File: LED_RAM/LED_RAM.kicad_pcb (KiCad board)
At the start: 2 copper layers, 196.3 x 403.9 mm, 91 parts, among them J1 DIN, J10 USB_C_Receptacle_PowerOnly_6P, J12 Conn_01x08_Pin, J13 Conn_01x22_Pin, J14 Conn_01x22_Pin, J15 Conn_01x22_Pin, J16 Conn_01x22_Pin, J2 5V, J3 GND, J4 DOUT, J5 Conn_01x05_Pin, J6 Conn_01x10_Pin, J7 DIN, J8 GND, J9 5V, U1 ER_OLEDM0.91_1x-I2C, U2 ER_OLEDM0.91_1x-I2C, U5 TXS0108EPW, U6 TXS0108EPW, U7 TXS0108EPW

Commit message: Add files via upload
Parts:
- moved D33 290.1 mm to (-33.7, 25.3)
- moved D34 290.1 mm to (-33.7, 50.3)
- moved D35 290.1 mm to (-33.7, 75.3)
- moved D38 290.1 mm to (-33.7, 150.3)
- moved D39 290.1 mm to (-33.7, 175.3)
- moved D40 290.1 mm to (-33.7, 200.3)
- moved J1 290.1 mm to (-46.9, 204.6)
- moved J2 290.1 mm to (46.3, 25.1)
- moved J4 290.1 mm to (-50.5, 204.6)
- moved D1 290.1 mm to (-133.4, 25.2)
- moved D10 290.1 mm to (-108.9, 50.1)
- moved D11 290.1 mm to (-108.9, 75.1)
- moved D12 290.1 mm to (-108.9, 100.1)
- moved D13 290.1 mm to (-108.9, 125.1)
- moved D14 290.1 mm to (-108.9, 150.1)
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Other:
- board size 196.3 x 403.9 mm -> 400.6 x 200.2 mm
- board text added: "SOUP-A COOL LED CUBE :D for FallOut 2026"

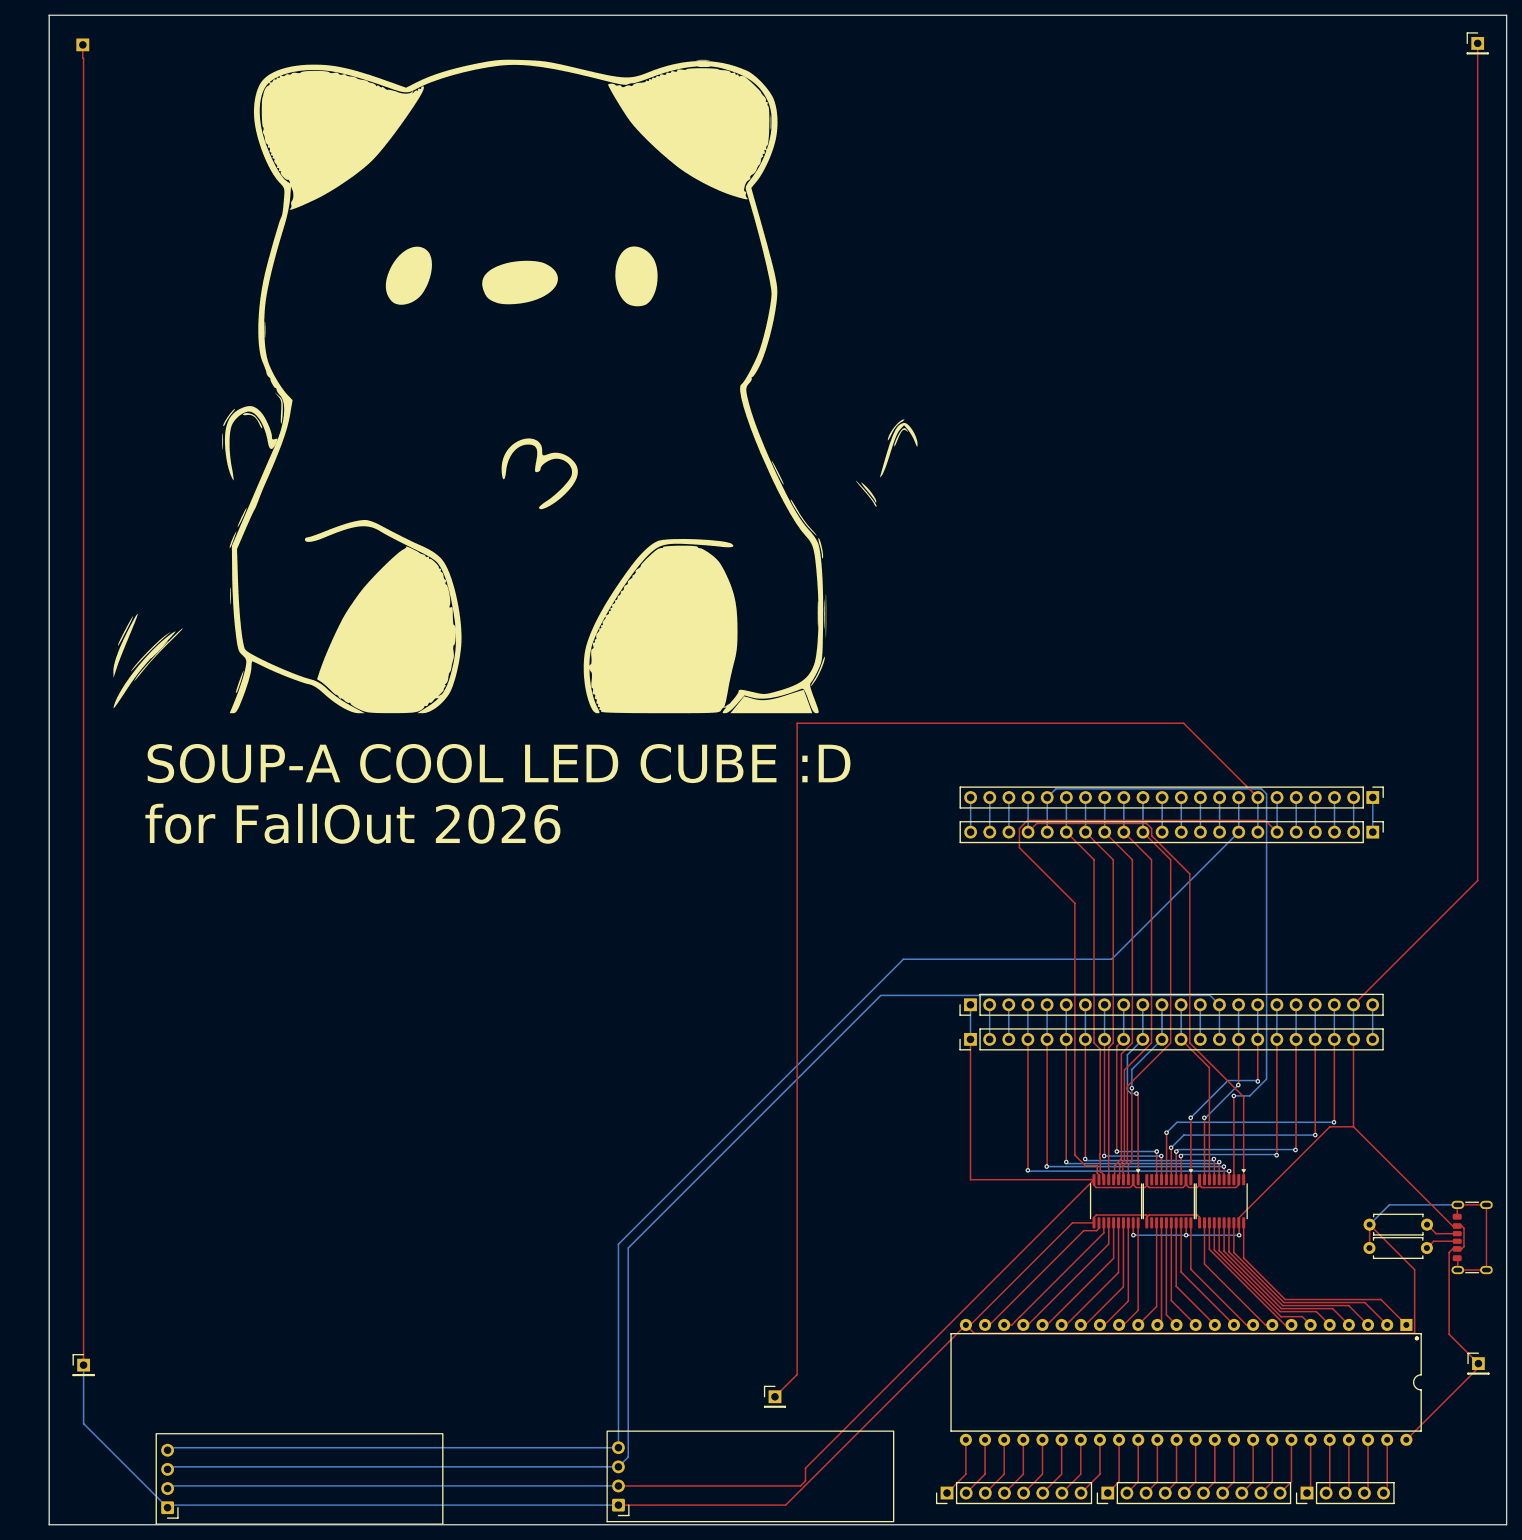
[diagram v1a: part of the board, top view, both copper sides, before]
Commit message: Add files via upload
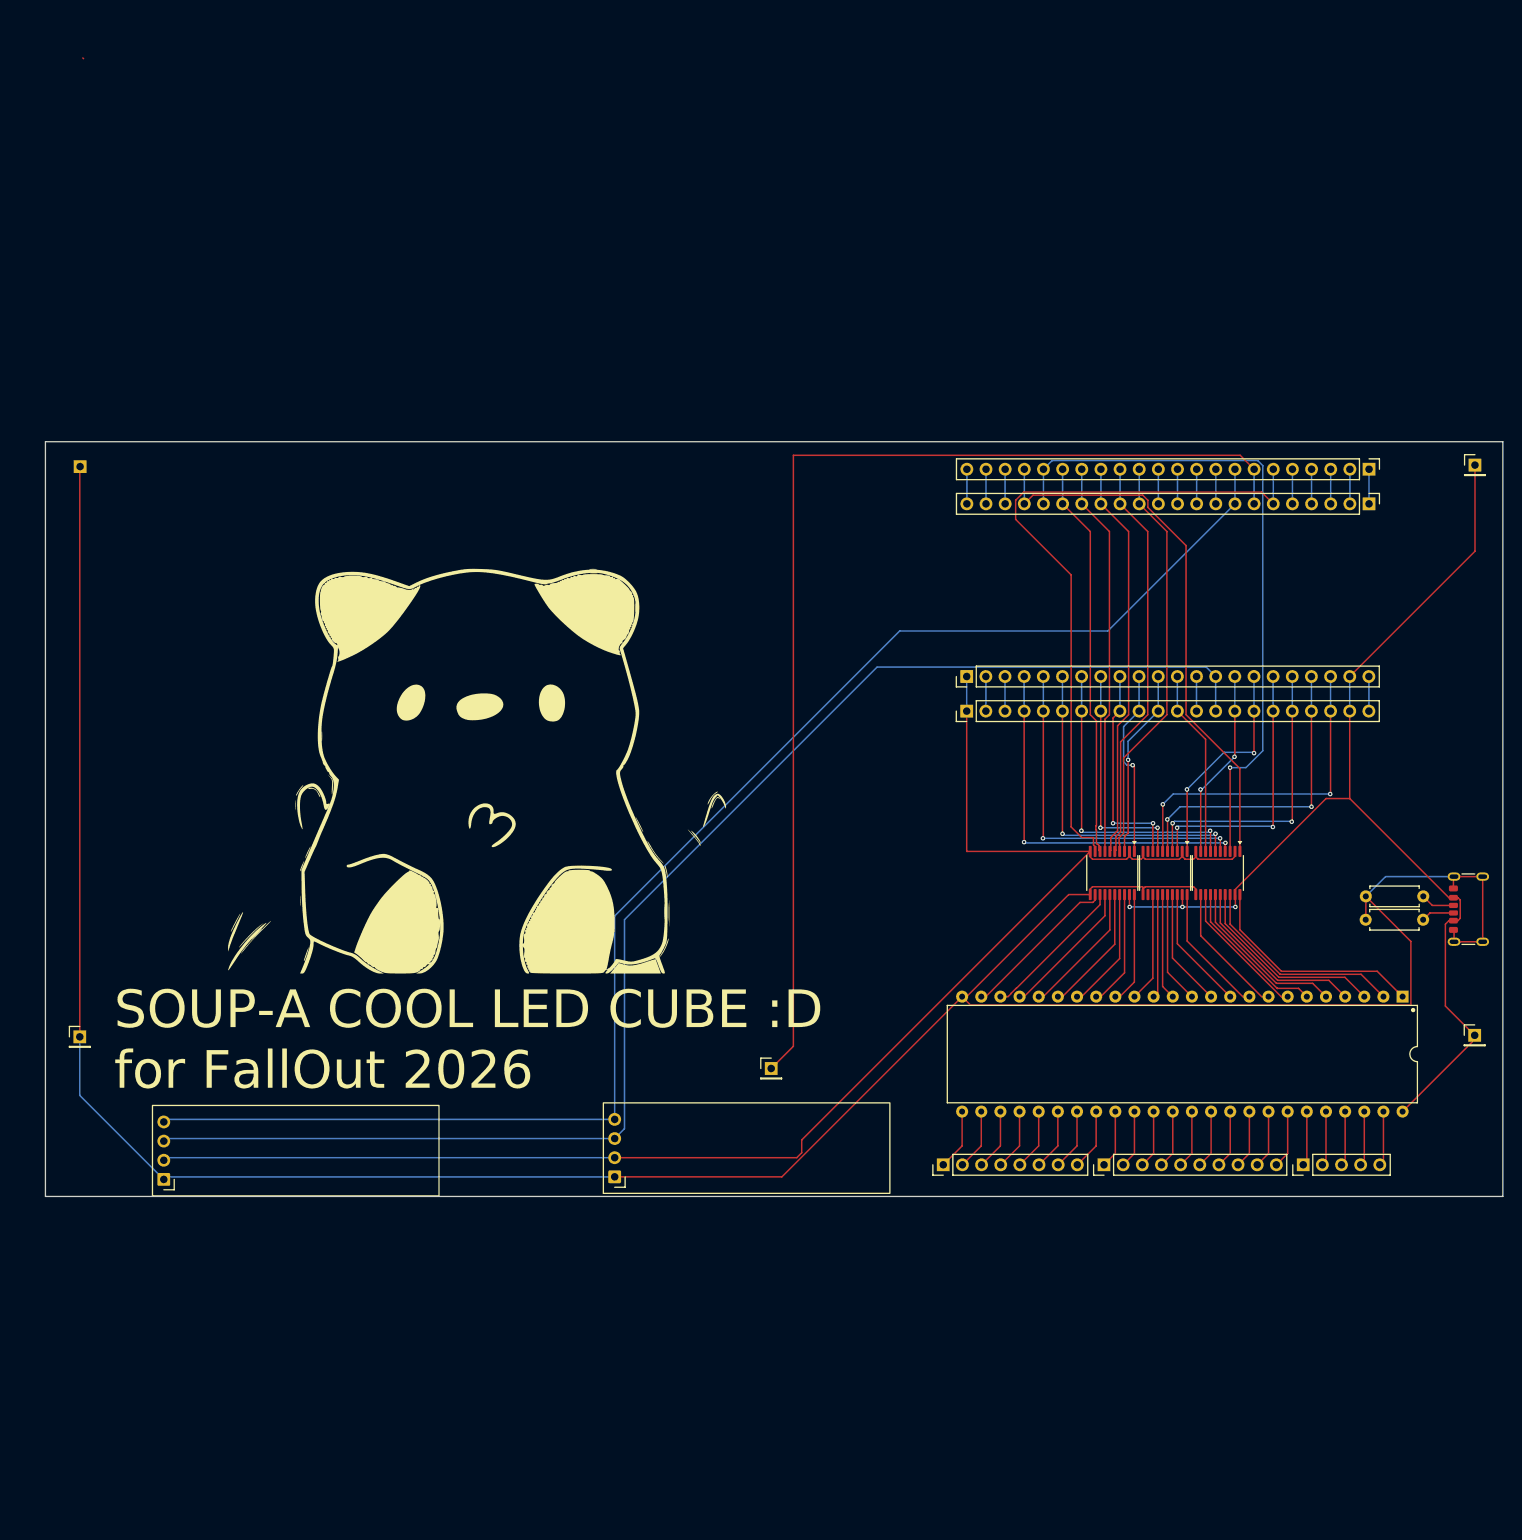
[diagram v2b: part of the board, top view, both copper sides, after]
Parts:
- moved J9 55.9 mm to (255.0, 79.8)
- moved ? 55.9 mm to (70.0, 80.0)
- moved J9 43.5 mm to (255.0, 155.4)
- moved U3 43.5 mm to (245.4, 150.3)
- moved J15 43.5 mm to (187.6, 112.4)
- moved J16 43.5 mm to (187.6, 107.8)
- moved J10 43.5 mm to (255.2, 138.7)
- moved J12 43.5 mm to (184.5, 172.6)
- moved J13 43.5 mm to (240.9, 80.3)
- moved J14 43.5 mm to (240.9, 84.9)
- moved J5 43.5 mm to (232.2, 172.6)
- moved J6 43.5 mm to (205.8, 172.6)
- moved J7 43.5 mm to (161.7, 159.8)
- moved J8 43.5 mm to (70.0, 155.6)
- moved R1 43.5 mm to (240.5, 137.0)
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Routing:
- net /5V: track 245.7 -> 146.3 mm
- net GND: track 2091.1 -> 1991.8 mm
- net Net-(J13-Pin_7): track 160.3 -> 149.0 mm
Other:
- board size 400.6 x 200.2 mm -> 400.1 x 184.2 mm
